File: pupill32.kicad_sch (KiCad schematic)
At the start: 50 parts, among them J1 HeaderR, J2 HeaderL, J3 USB_PINS, J4 SWD_HEADER, SW1 RST_BTN, SW2 BOOT_BTN, U1 SRV05-4, U2 PY32F030F18P6, U3 CH340N, U4 AMS1117-3.3, Y1 32.768 kHz, Y2 12M

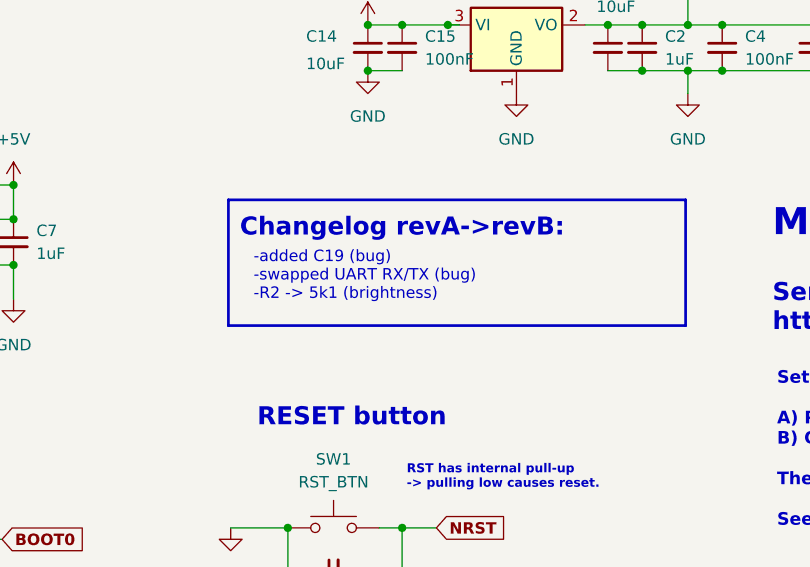
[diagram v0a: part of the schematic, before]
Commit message: schema changelog update
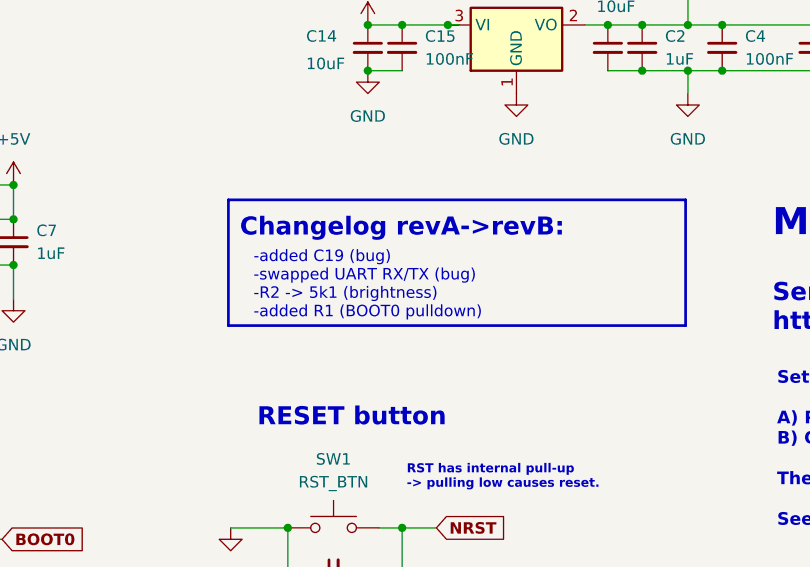
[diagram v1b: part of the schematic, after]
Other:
- note added: "-added C19 (bug) -swapped UART RX/TX (bug) -R2 -> 5k1 (brightness) -added R1 (BOOT0 pulldown)"
- note removed: "-added C19 (bug) -swapped UART RX/TX (bug) -R2 -> 5k1 (brightness)"
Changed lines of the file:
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@@
 		)
 	)
-	(text "-added C19 (bug)\n-swapped UART RX/TX (bug)\n-R2 -> 5k1 (brightness)"
+	(text "-added C19 (bug)\n-swapped UART RX/TX (bug)\n-R2 -> 5k1 (brightness)\n-added R1 (BOOT0 pulldown)"
 		(exclude_from_sim no)
-		(at 93.98 127 0)
+		(at 93.98 128.016 0)
 		(effects
 			(font
